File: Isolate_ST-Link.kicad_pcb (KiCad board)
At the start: 2 copper layers, 39 x 38 mm, 70 parts, among them J1 USB_OTG, J2 Conn_02x05_Odd_Even, J3 CONN_01X04, J4 CONN_01X02, J5 CONN_01X02, J6 GS2, Q1 BSS138, U1 MAU10x, U2 ADuM4160, U3 APE8865NR-33-HF-3, U4 STM32F103CBTx, Y1 Crystal

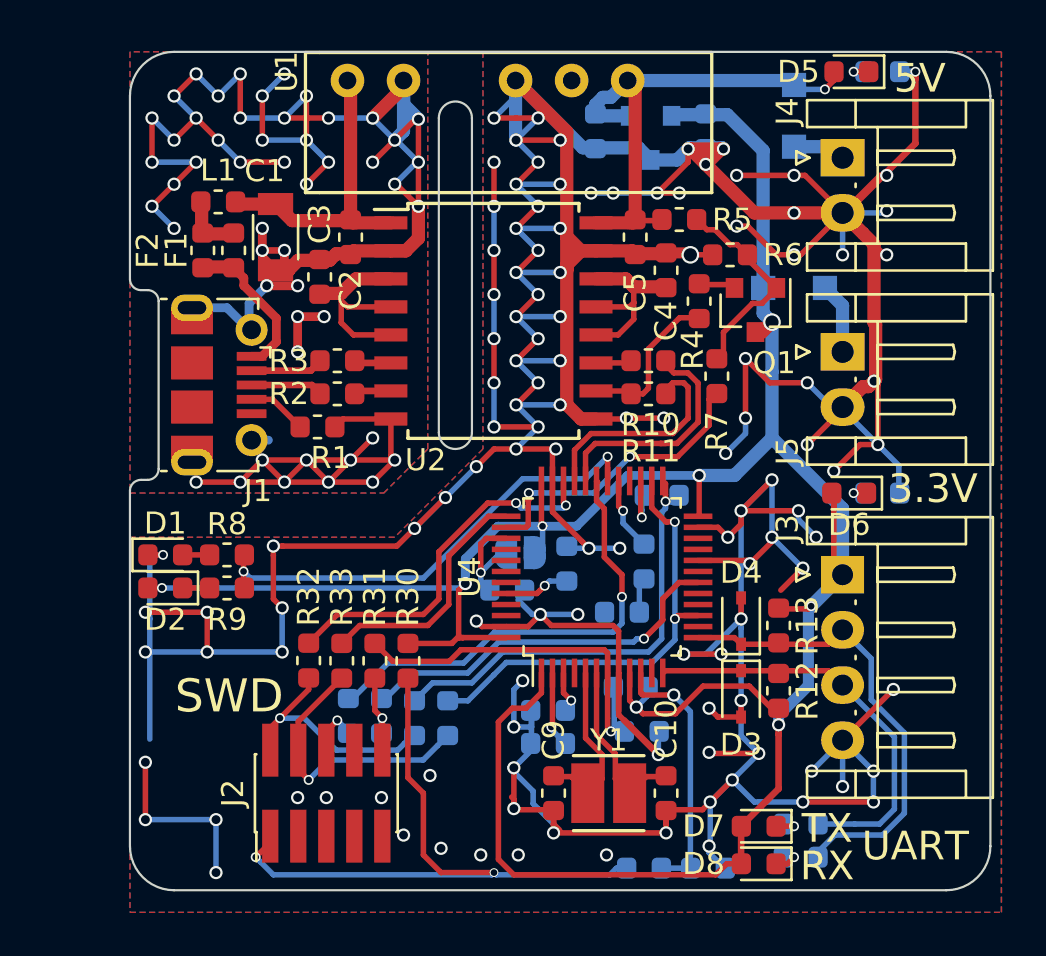
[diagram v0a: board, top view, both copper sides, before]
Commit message: 最低限の配線はできたんじゃね
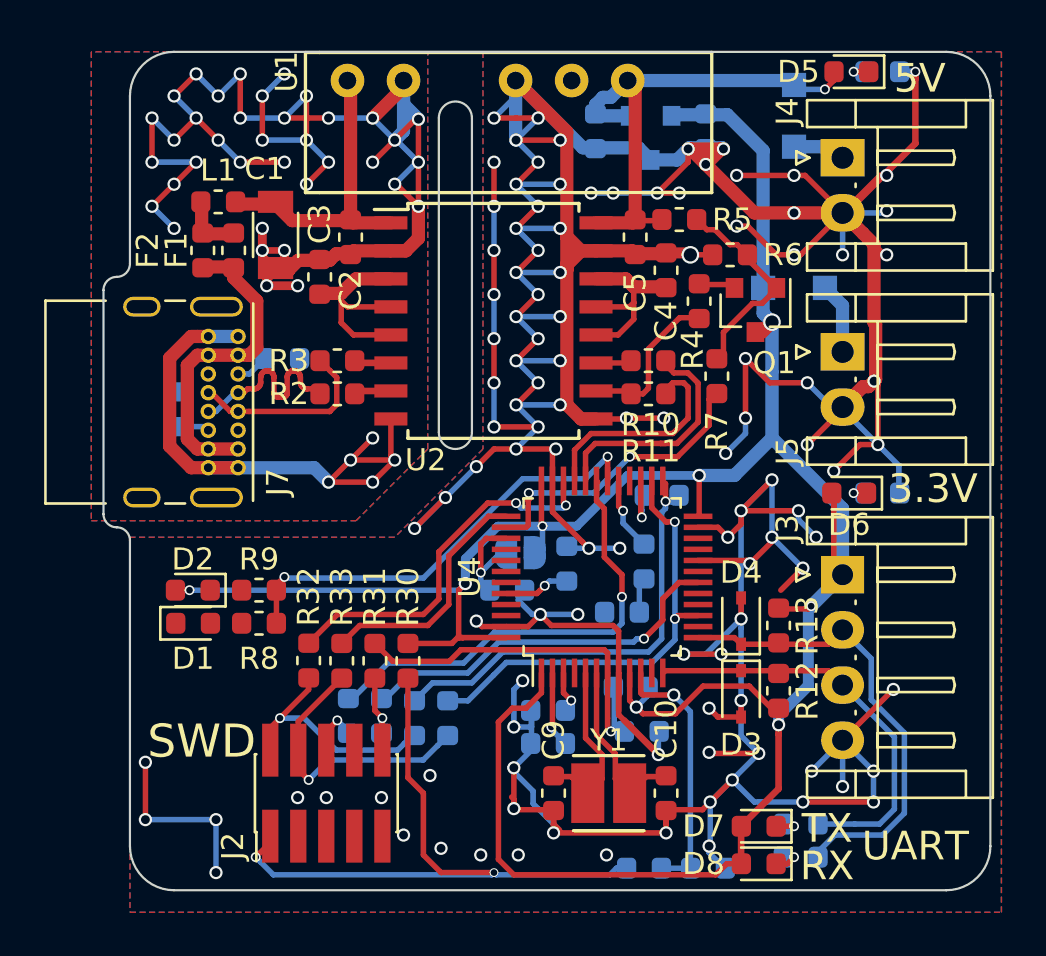
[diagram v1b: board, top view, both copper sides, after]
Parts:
- removed J1: USB_OTG, Connector_USB:USB_Micro-B_Molex-105017-0001
- added J7: USB_C_Receptacle_USB2.0, Connector_USB:USB_C_Receptacle_GCT_USB4085, F.Cu at (158.4, 62.9)
- added R35: 5.1k, Resistor_SMD:R_0603_1608Metric, B.Cu at (160.4, 63.9)
- R1: value 100k -> 5.1k; moved to B.Cu
- moved R1 6.35 mm to (155.7, 66.2), turned to 270 degrees
- moved R8 3.42 mm to (159.3, 75.9)
- moved D1 3.35 mm to (156.4, 75.9)
- moved R9 1.45 mm to (159.3, 74.4)
- moved D2 1.25 mm to (156.3, 74.4)
- moved C1 0.10 mm to (160.1, 58.3)
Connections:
- net Net-(R2-Pad2) renamed /UD+
- net Net-(R3-Pad1) renamed /UD-
- R1 pad 1: Net-(J1-Pad4) -> GNDPWR
- R1 pad 2: GNDPWR -> Net-(J7-PadB5)
- R2 pad 1: Net-(J1-Pad3) -> /DIN_+
- R3 pad 2: Net-(J1-Pad2) -> /DIN_-
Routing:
- net GND: track 351.7 -> 319.7 mm, vias 120 -> 112
- net GNDPWR: track 113.8 -> 103.0 mm, vias 50 -> 42
- net /DIN_+: track 0.00 -> 8.68 mm
- net /DIN_-: track 0.00 -> 8.61 mm
- net Net-(F1-Pad2): track 6.96 -> 14.8 mm
- net Net-(J1-Pad2): track 6.72 -> 0.00 mm
- net Net-(J1-Pad3): track 6.68 -> 0.00 mm
- net Net-(J1-Pad4): track 2.72 -> 0.00 mm
- net Net-(J7-PadA5): track 0.00 -> 1.50 mm
- net Net-(J7-PadB5): track 0.00 -> 1.42 mm
- net Net-(D2-Pad1): track 1.25 -> 0.00 mm
- net Net-(D1-Pad2): track 1.25 -> 0.00 mm
- net +3V3: track 124.3 -> 123.1 mm
- net /MCU/LED_STLINK: track 21.5 -> 20.3 mm
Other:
- board size 39 x 38 mm -> 40.2 x 38 mm
- board text removed: "Isolate_ST-Link"
